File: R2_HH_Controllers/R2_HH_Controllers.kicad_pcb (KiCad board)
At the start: 4 copper layers, 30.4 x 82.4 mm, 55 parts, among them IC1 E22-900M22S, J2 USB4105-GF-A, J3 S2B-PH-SM4-TB_LF__SN_, SW1 SW_Push, SW10 Reset, SW12 Boot, SW2 SW_Push, SW3 SW_Push, SW4 SW_Push, SW5 SW_Push, SW6 SW_Push, SW7 SW_Push, SW8 SW_Push, SW9 PCM12SMTR, U1 ESP32-S3-WROOM-1, U2 USBLC6-2SC6, U3 BQ24074RGT, U5 AP2112K-3.3

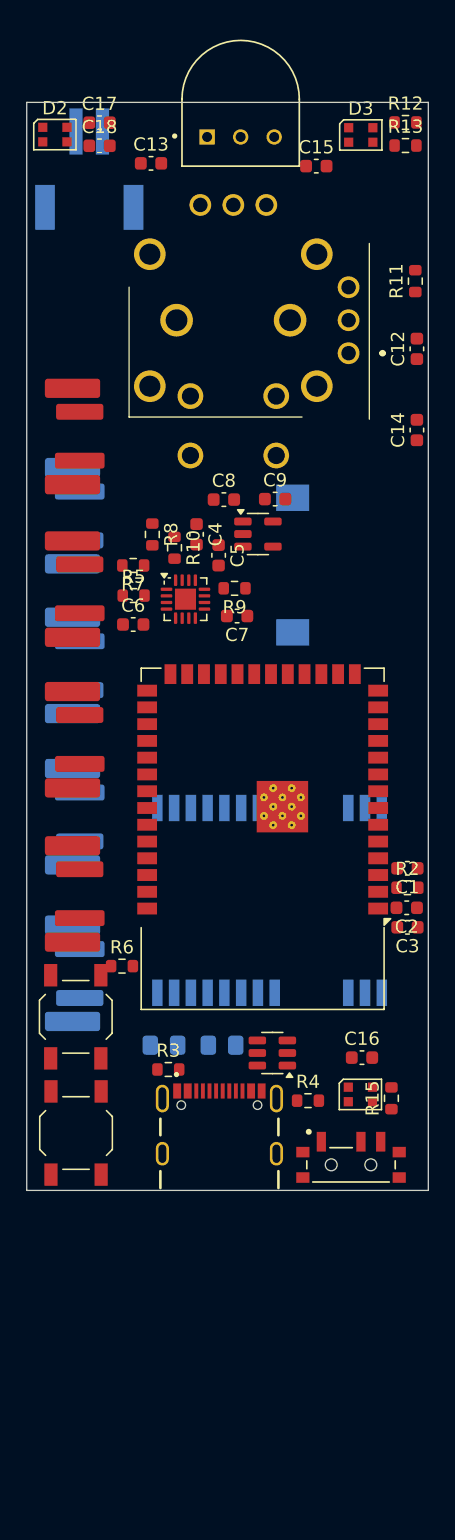
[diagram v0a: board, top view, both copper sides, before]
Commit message: updates
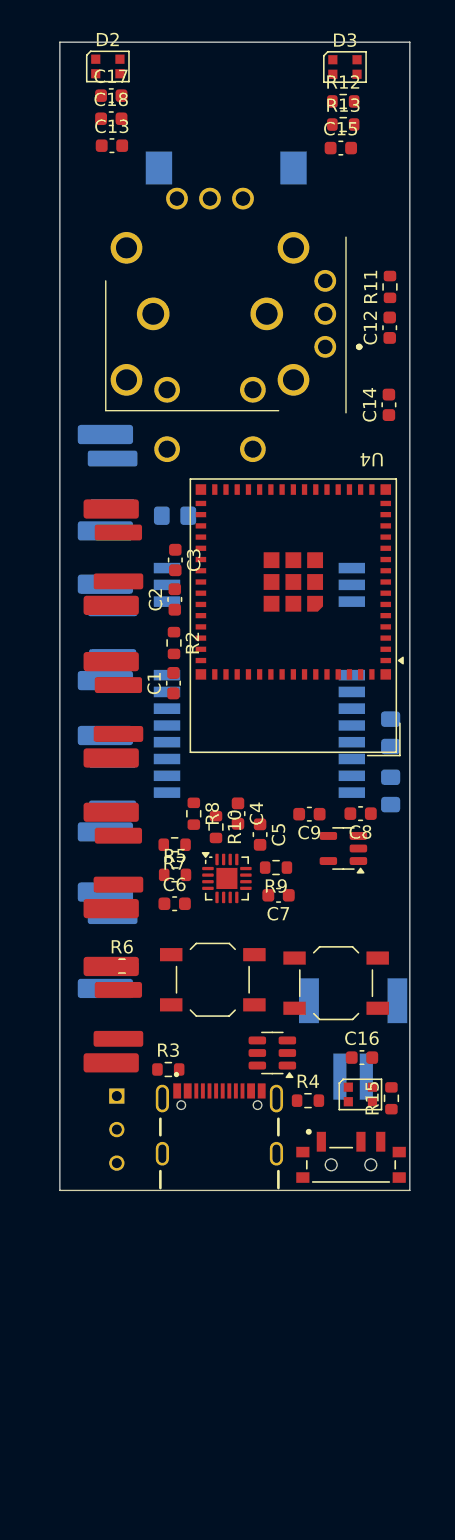
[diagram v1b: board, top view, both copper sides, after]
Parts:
- removed U1: ESP32-S3-WROOM-1, RF_Module:ESP32-S3-WROOM-1
- added R14: DNP, Resistor_SMD:R_0805_2012Metric_Pad1.20x1.40mm_HandSolder, B.Cu at (190.5, 60.8)
- added U4: ESP32-S3-MINI-1, RF_Module:ESP32-S2-MINI-1, F.Cu at (199.4, 68.4)
- R1: moved to B.Cu
- moved R1 79.0 mm to (183.2, 107.3), turned to -90 degrees
- moved J3 74.3 mm to (203.9, 103.3), turned to 0 degrees
- moved E1 35.9 mm to (194.3, 29.9), turned to 180 degrees
- moved C3 32.9 mm to (190.5, 64.2), turned to -90 degrees
- moved C2 29.2 mm to (190.4, 67.2), turned to 90 degrees
- moved C11 26.9 mm to (206.8, 77.3), turned to -90 degrees
- moved C8 25.9 mm to (204.5, 83.4), turned to 180 degrees
- moved C10 25.8 mm to (206.8, 81.7), turned to 90 degrees
- moved R2 25.6 mm to (190.4, 70.5), turned to -90 degrees
- moved U5 24.7 mm to (203.2, 86.0), turned to 180 degrees
- moved C9 24.0 mm to (200.6, 83.4), turned to 180 degrees
- moved SW10 22.7 mm to (202.7, 96.2), turned to 0 degrees
- moved C1 22.6 mm to (190.3, 73.5), turned to 90 degrees
- moved C4 21.4 mm to (195.2, 83.4)
- moved C6 21.4 mm to (190.4, 90.2)
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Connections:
- E1 pad 1: Net-(IC1-ANT) -> Net-(E1-Pad1)
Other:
- board size 30.4 x 82.4 mm -> 26.5 x 87 mm

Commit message: sabe
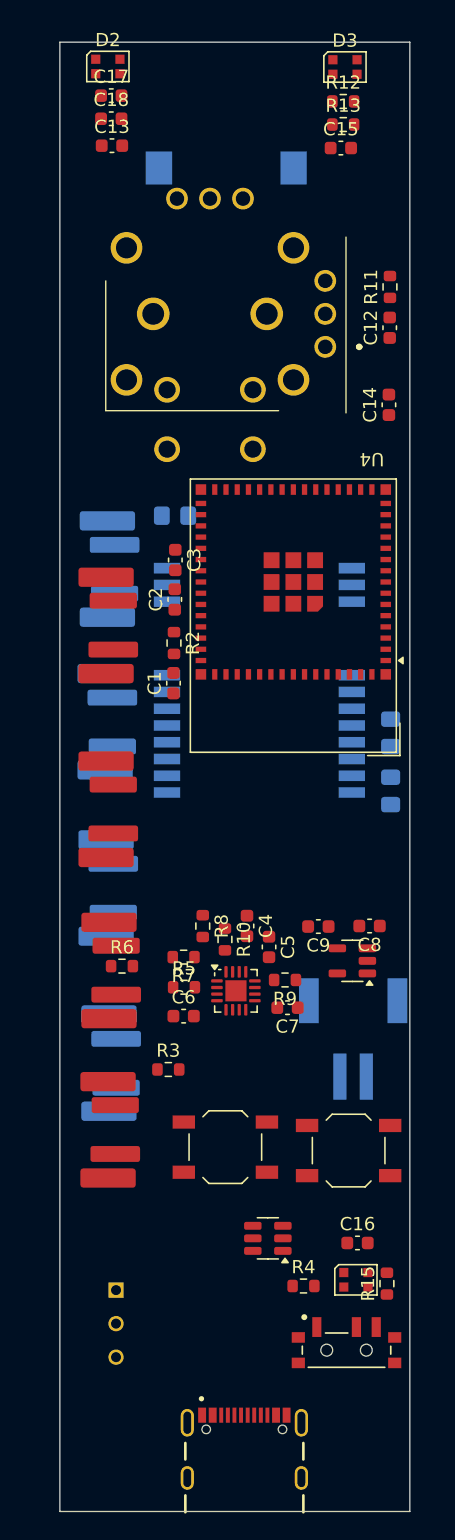
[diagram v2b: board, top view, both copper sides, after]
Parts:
- moved J2 24.6 mm to (195.7, 133.7)
- moved R1 14.7 mm to (183.1, 122.0)
- moved D1 14.0 mm to (204.2, 118.7)
- moved R4 14.0 mm to (200.2, 119.2)
- moved SW9 14.0 mm to (203.4, 124.0)
- moved U2 14.0 mm to (197.5, 115.6)
- moved C16 14.0 mm to (204.3, 115.9)
- moved R15 14.0 mm to (206.5, 119.0)
- moved SW12 12.7 mm to (194.3, 108.7)
- moved SW10 12.7 mm to (203.6, 108.9)
- moved SW8 9.30 mm to (182.4, 102.3)
- moved SW4 8.73 mm to (182.3, 107.3)
- moved C5 8.54 mm to (197.6, 93.5)
- moved C6 8.54 mm to (191.1, 98.7)
- moved C8 8.54 mm to (205.2, 91.9)
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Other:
- board size 26.5 x 87 mm -> 26.5 x 111.3 mm
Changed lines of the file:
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@@
 	(footprint "Resistor_SMD:R_0603_1608Metric"
 		(layer "F.Cu")
-		(at 206.85 104.95 90)
+		(at 206.51 118.99 90)
 		(descr "Resistor SMD 0603 (1608 Metric), square (rectangular) end terminal, IPC-7351 nominal, (Body size source: IPC-SM-782 page 72, https://www.pcb-3d.com/wordpress/wp-content/uploads/ipc-sm-782a_amendment_1_and_2.pdf), generated with kicad-footprint-generator")
 		(tags "resistor")
@@
 	(footprint "Capacitor_SMD:C_0603_1608Metric"
 		(layer "F.Cu")
-		(at 204.62 101.87)
+		(at 204.28 115.91)
 		(descr "Capacitor SMD 0603 (1608 Metric), square (rectangular) end terminal, IPC-7351 nominal, (Body size source: IPC-SM-782 page 76, https://www.pcb-3d.com/wordpress/wp-content/uploads/ipc-sm-782a_amendment_1_and_2.pdf), generated with kicad-footprint-generator")
 		(tags "capacitor")
@@
 	(footprint "Capacitor_SMD:C_0603_1608Metric"
 		(layer "F.Cu")
-		(at 200.635 83.4275 180)
+		(at 201.315 91.94 180)
 		(descr "Capacitor SMD 0603 (1608 Metric), square (rectangular) end terminal, IPC-7351 nominal, (Body size source: IPC-SM-782 page 76, https://www.pcb-3d.com/wordpress/wp-content/uploads/ipc-sm-782a_amendment_1_and_2.pdf), generated with kicad-footprint-generator")
 		(tags "capacitor")
@@
 	(footprint "01-Custom:TL3360CF185Q"
 		(layer "F.Cu")
-		(at 182.59 98.616 90)
+		(at 182.35 107.34 90)
 		(property "Reference" "SW4"
 			(at 0 -3 90)
@@
 	(footprint "Button_Switch_SMD:SW_SPST_TL3342"
 		(layer "F.Cu")
-		(at 193.32 95.97 180)
+		(at 194.27 108.65 180)
 		(descr "Low-profile SMD Tactile Switch, https://www.e-switch.com/system/asset/product_line/data_sheet/165/TL3342.pdf")
 		(tags "SPST Tactile Switch")
@@
 	(footprint "01-Custom:GCT_USB4105-GF-A"
 		(layer "F.Cu")
-		(at 193.82 109.15)
+		(at 195.71 133.71)
 		(property "Reference" "J2"
 			(at -1.825 -8.635 0)
@@
 	(footprint "01-Custom:TL3360CF185Q"
 		(layer "F.Cu")
-		(at 182.59 75.523 90)
+		(at 182.2 83.06 90)
 		(property "Reference" "SW2"
 			(at 0 -3 90)
@@
 	(footprint "Capacitor_SMD:C_0603_1608Metric"
 		(layer "F.Cu")
-		(at 195.23 83.385 -90)
+		(at 195.91 91.8975 -90)
 		(descr "Capacitor SMD 0603 (1608 Metric), square (rectangular) end terminal, IPC-7351 nominal, (Body size source: IPC-SM-782 page 76, https://www.pcb-3d.com/wordpress/wp-content/uploads/ipc-sm-782a_amendment_1_and_2.pdf), generated with kicad-footprint-generator")
 		(tags "capacitor")
@@
 	(footprint "Package_TO_SOT_SMD:SOT-23-6"
 		(layer "F.Cu")
-		(at 197.83 101.52 180)
+		(at 197.49 115.56 180)
 		(descr "SOT, 6 Pin (JEDEC MO-178 Var AB https://www.jedec.org/document_search?search_api_views_fulltext=MO-178), generated with kicad-footprint-generator ipc_gullwing_generator.py")
 		(tags "SOT TO_SOT_SMD")
@@
 	(footprint "Capacitor_SMD:C_0603_1608Metric"
 		(layer "F.Cu")
-		(at 190.43 90.215)
+		(at 191.11 98.7275)
 		(descr "Capacitor SMD 0603 (1608 Metric), square (rectangular) end terminal, IPC-7351 nominal, (Body size source: IPC-SM-782 page 76, https://www.pcb-3d.com/wordpress/wp-content/uploads/ipc-sm-782a_amendment_1_and_2.pdf), generated with kicad-footprint-generator")
 		(tags "capacitor")
@@
 	(footprint "01-Custom:SW_PCM12SMTR"
 		(layer "F.Cu")
-		(at 203.79 109.99)
+		(at 203.45 124.03)
 		(property "Reference" "SW9"
 			(at -0.635 -4.699 0)
@@
 	(footprint "Capacitor_SMD:C_0603_1608Metric"
 		(layer "F.Cu")
-		(at 204.515 83.3875 180)
+		(at 205.195 91.9 180)
 		(descr "Capacitor SMD 0603 (1608 Metric), square (rectangular) end terminal, IPC-7351 nominal, (Body size source: IPC-SM-782 page 76, https://www.pcb-3d.com/wordpress/wp-content/uploads/ipc-sm-782a_amendment_1_and_2.pdf), generated with kicad-footprint-generator")
 		(tags "capacitor")
@@
 	(footprint "Resistor_SMD:R_0603_1608Metric"
 		(layer "F.Cu")
-		(at 193.56 84.405 -90)
+		(at 194.24 92.9175 -90)
 		(descr "Resistor SMD 0603 (1608 Metric), square (rectangular) end terminal, IPC-7351 nominal, (Body size source: IPC-SM-782 page 72, https://www.pcb-3d.com/wordpress/wp-content/uploads/ipc-sm-782a_amendment_1_and_2.pdf), generated with kicad-footprint-generator")
 		(tags "resistor")
@@
 	(footprint "Package_TO_SOT_SMD:SOT-23-5"
 		(layer "F.Cu")
-		(at 203.2125 86.0275 180)
+		(at 203.8925 94.54 180)
 		(descr "SOT, 5 Pin (JEDEC MO-178 Var AA https://www.jedec.org/document_search?search_api_views_fulltext=MO-178), generated with kicad-footprint-generator ipc_gullwing_generator.py")
 		(tags "SOT TO_SOT_SMD")
@@
 	(footprint "Resistor_SMD:R_0603_1608Metric"
 		(layer "F.Cu")
-		(at 190.46 88.025)
+		(at 191.14 96.5375)
 		(descr "Resistor SMD 0603 (1608 Metric), square (rectangular) end terminal, IPC-7351 nominal, (Body size source: IPC-SM-782 page 72, https://www.pcb-3d.com/wordpress/wp-content/uploads/ipc-sm-782a_amendment_1_and_2.pdf), generated with kicad-footprint-generator")
 		(tags "resistor")
@@
 	(footprint "LED_SMD:LED_WS2812B-2020_PLCC4_2.0x2.0mm"
 		(layer "F.Cu")
-		(at 204.5 104.66)
+		(at 204.16 118.7)
 		(descr "2.0mm x 2.0mm Addressable RGB LED NeoPixel Nano, 12 mA, https://cdn-shop.adafruit.com/product-files/4684/4684_WS2812B-2020_V1.3_EN.pdf")
 		(tags "LED RGB NeoPixel Nano PLCC-4 2020")
@@
 	(footprint "Button_Switch_SMD:SW_SPST_TL3342"
 		(layer "F.Cu")
-		(at 202.66 96.23)
+		(at 203.61 108.91)
 		(descr "Low-profile SMD Tactile Switch, https://www.e-switch.com/system/asset/product_line/data_sheet/165/TL3342.pdf")
 		(tags "SPST Tactile Switch")
@@
 	(footprint "Resistor_SMD:R_0603_1608Metric"
 		(layer "F.Cu")
-		(at 200.53 105.13)
+		(at 200.19 119.17)
 		(descr "Resistor SMD 0603 (1608 Metric), square (rectangular) end terminal, IPC-7351 nominal, (Body size source: IPC-SM-782 page 72, https://www.pcb-3d.com/wordpress/wp-content/uploads/ipc-sm-782a_amendment_1_and_2.pdf), generated with kicad-footprint-generator")
 		(tags "resistor")
@@
 	(footprint "Capacitor_SMD:C_0603_1608Metric"
 		(layer "F.Cu")
-		(at 196.9 84.975 -90)
+		(at 197.58 93.4875 -90)
 		(descr "Capacitor SMD 0603 (1608 Metric), square (rectangular) end terminal, IPC-7351 nominal, (Body size source: IPC-SM-782 page 76, https://www.pcb-3d.com/wordpress/wp-content/uploads/ipc-sm-782a_amendment_1_and_2.pdf), generated with kicad-footprint-generator")
 		(tags "capacitor")
@@
 	(footprint "Package_DFN_QFN:VQFN-16-1EP_3x3mm_P0.5mm_EP1.6x1.6mm"
 		(layer "F.Cu")
-		(at 194.39 88.2975)
+		(at 195.07 96.81)
 		(descr "VQFN, 16 Pin (http://www.ti.com/lit/ds/symlink/cdclvp1102.pdf#page=28), generated with kicad-footprint-generator ipc_noLead_generator.py")
 		(tags "VQFN NoLead")
@@
 	(footprint "01-Custom:TL3360CF185Q"
 		(layer "F.Cu")
-		(at 182.59 86.933 90)
+		(at 182.42 95.27 90)
 		(property "Reference" "SW3"
 			(at 0 -3 90)
@@
 	(footprint "Capacitor_SMD:C_0603_1608Metric"
 		(layer "F.Cu")
-		(at 198.3 89.575 180)
+		(at 198.98 98.0875 180)
 		(descr "Capacitor SMD 0603 (1608 Metric), square (rectangular) end terminal, IPC-7351 nominal, (Body size source: IPC-SM-782 page 76, https://www.pcb-3d.com/wordpress/wp-content/uploads/ipc-sm-782a_amendment_1_and_2.pdf), generated with kicad-footprint-generator")
 		(tags "capacitor")
@@
 	(footprint "Resistor_SMD:R_0603_1608Metric"
 		(layer "F.Cu")
-		(at 198.11 87.475 180)
+		(at 198.79 95.9875 180)
 		(descr "Resistor SMD 0603 (1608 Metric), square (rectangular) end terminal, IPC-7351 nominal, (Body size source: IPC-SM-782 page 72, https://www.pcb-3d.com/wordpress/wp-content/uploads/ipc-sm-782a_amendment_1_and_2.pdf), generated with kicad-footprint-generator")
 		(tags "resistor")
@@
 	(footprint "Resistor_SMD:R_0603_1608Metric"
 		(layer "F.Cu")
-		(at 191.88 83.395 -90)
+		(at 192.56 91.9075 -90)
 		(descr "Resistor SMD 0603 (1608 Metric), square (rectangular) end terminal, IPC-7351 nominal, (Body size source: IPC-SM-782 page 72, https://www.pcb-3d.com/wordpress/wp-content/uploads/ipc-sm-782a_amendment_1_and_2.pdf), generated with kicad-footprint-generator")
 		(tags "resistor")
@@
 	(footprint "Resistor_SMD:R_0603_1608Metric"
 		(layer "F.Cu")
-		(at 190.43 85.745 180)
+		(at 191.11 94.2575 180)
 		(descr "Resistor SMD 0603 (1608 Metric), square (rectangular) end terminal, IPC-7351 nominal, (Body size source: IPC-SM-782 page 72, https://www.pcb-3d.com/wordpress/wp-content/uploads/ipc-sm-782a_amendment_1_and_2.pdf), generated with kicad-footprint-generator")
 		(tags "resistor")
@@
 	(footprint "01-Custom:TL3360CF185Q"
 		(layer "F.Cu")
-		(at 182.59 63.963 90)
+		(at 182.2 69.13 90)
 		(property "Reference" "SW1"
 			(at 0 -10.86625 270)
@@
 	(footprint "01-Custom:TL3360CF185Q"
 		(layer "B.Cu")
-		(at 182.15 69.66 -90)
+		(at 182.13 76.43 -90)
 		(property "Reference" "SW6"
 			(at 0 3 90)
@@
 	(footprint "01-Custom:TL3360CF185Q"
 		(layer "B.Cu")
-		(at 182.15 92.98 -90)
+		(at 182.42 102.28 -90)
 		(property "Reference" "SW8"
 			(at 0 3 90)
@@
 	(footprint "01-Custom:TL3360CF185Q"
 		(layer "B.Cu")
-		(at 182.15 58.32 -90)
+		(at 182.3 64.86 -90)
 		(property "Reference" "SW5"
 			(at 0 3 90)
@@
 	(footprint "01-Custom:TL3360CF185Q"
 		(layer "B.Cu")
-		(at 182.15 81.12 -90)
+		(at 182.2 89.02 -90)
 		(property "Reference" "SW7"
 			(at -0.64 -0.7 270)
@@
 	(footprint "01-Custom:TRIM_3352T-1-103LF"
 		(layer "B.Cu")
-		(at 183.18 107.32 -90)
+		(at 183.12 122.02 -90)
 		(property "Reference" "R1"
 			(at -0.625 5.435 90)
@@
 	(gr_rect
 		(start 181.735 24.95)
-		(end 208.245 111.93)
+		(end 208.245 136.25)
 		(stroke
 			(width 0.05)
@@
 		(min_thickness 0.25)
 		(filled_areas_thickness no)
-		(fill yes
+		(fill
 			(thermal_gap 0.5)
 			(thermal_bridge_width 0.5)
@@
 		(polygon
 			(pts
-				(xy 176.88 24.42) (xy 176.7 24.24) (xy 210.89 24.05) (xy 209.6 125.34) (xy 174.49 125.16)
+				(xy 176.88 24.42) (xy 176.7 24.24) (xy 210.89 24.05) (xy 209.05 137.36) (xy 177.98 137.74)
 			)
 		)
